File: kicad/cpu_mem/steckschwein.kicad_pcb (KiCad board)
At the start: 2 copper layers, 160 x 100.3 mm, 33 parts, among them P1 CONN_02X04, P3 CONN_01X03, P4 CONN_02X02, P5 CONN_02X25, SW1 SW_PUSH, U1 W65C02SP, U2 LM555N, U3 74HCT00, U4 74LS393, U5 GAL22V10, U6 28C256, U7 HM62256BLP-7, U8 HM62256BLP-7, U9 74LS139, X1 OSC

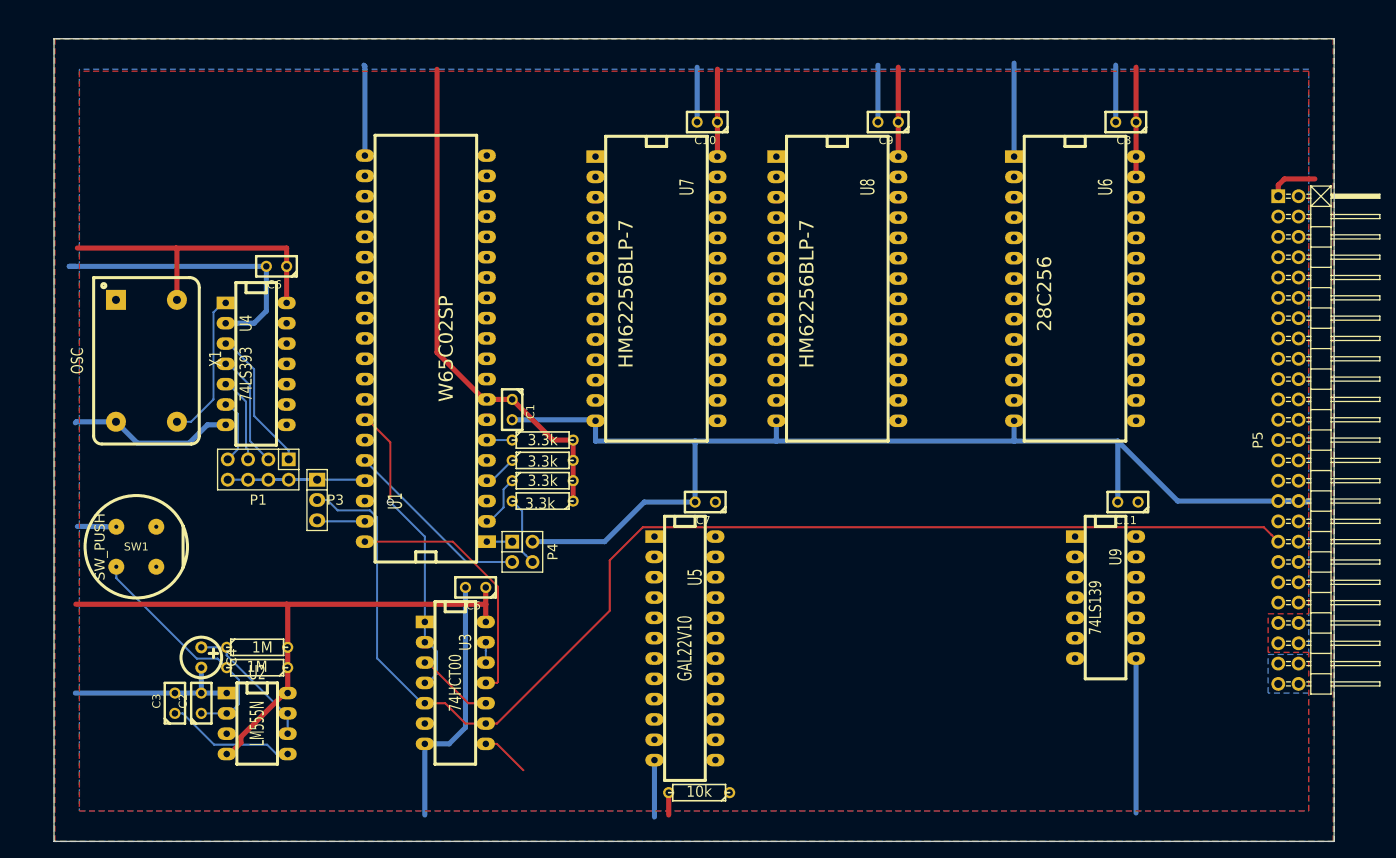
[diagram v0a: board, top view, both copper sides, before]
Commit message: new with new empty pcb
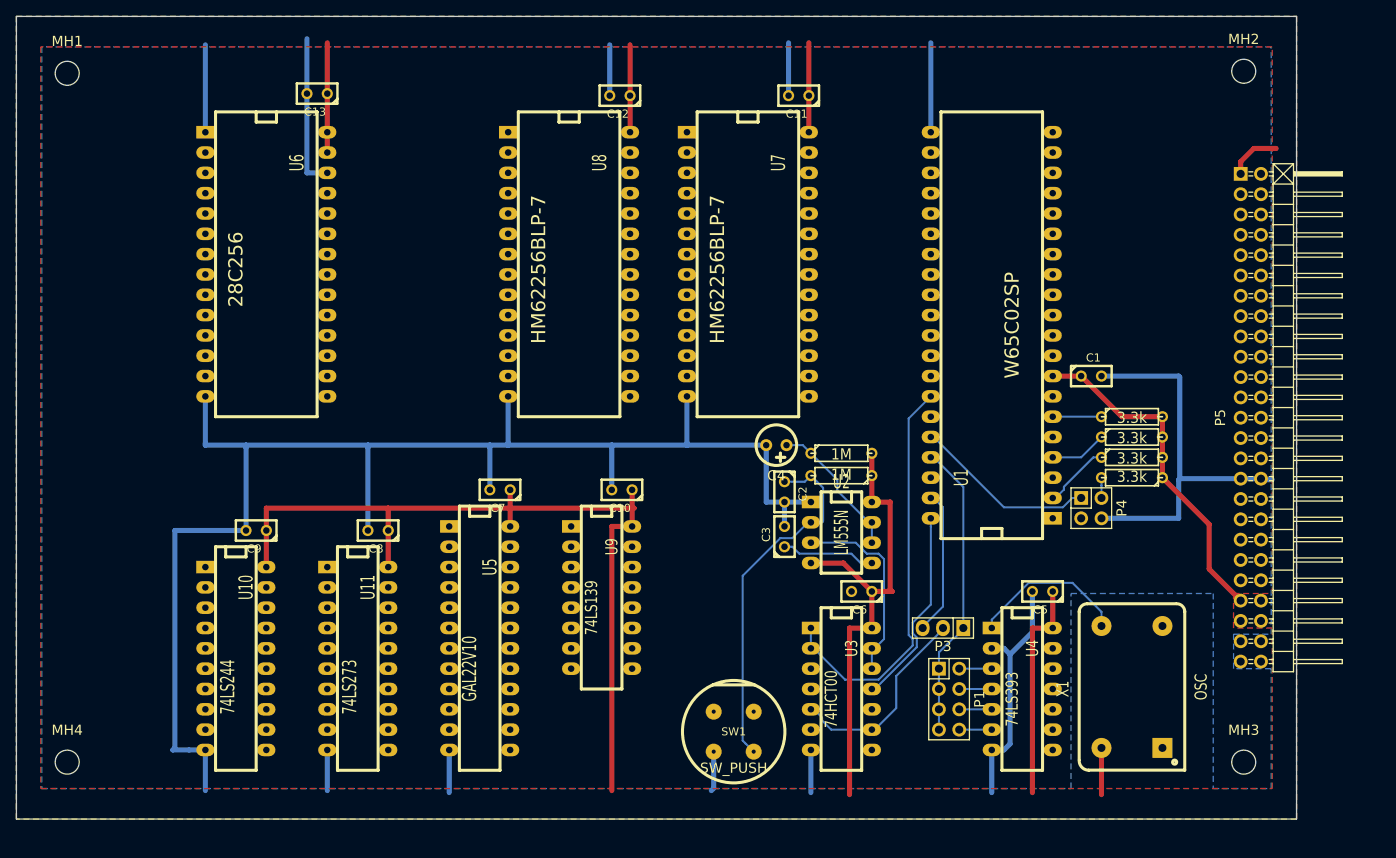
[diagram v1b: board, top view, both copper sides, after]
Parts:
- removed R8: 10k, Discret:R3
- added C12: 100n, Discret:C1, F.Cu at (137.7, 55.6)
- added C13: 100n, Discret:C1, F.Cu at (99.8, 55.4)
- added MH1: MountingHole_3mm_RevA_Date21Jun2010, Mounting_Holes:MountingHole_3mm, F.Cu at (68.6, 52.8)
- added MH2: MountingHole_3mm_RevA_Date21Jun2010, Mounting_Holes:MountingHole_3mm, F.Cu at (215.6, 52.6)
- added MH3: MountingHole_3mm_RevA_Date21Jun2010, Mounting_Holes:MountingHole_3mm, F.Cu at (215.6, 138.9)
- added MH4: MountingHole_3mm_RevA_Date21Jun2010, Mounting_Holes:MountingHole_3mm, F.Cu at (68.6, 138.9)
- added U10: 74LS244, Sockets_DIP:DIP-20__300_ELL, F.Cu at (89.7, 126.0)
- added U11: 74LS273, Sockets_DIP:DIP-20__300_ELL, F.Cu at (104.9, 126.0)
- U9: footprint Sockets_DIP:DIP-14__300_ELL -> Sockets_DIP:DIP-16__300_ELL
- moved X1 129.8 mm to (201.7, 129.5), turned to 90 degrees
- moved C8 106.5 mm to (107.4, 110.0)
- moved U4 104.0 mm to (188.0, 129.8)
- moved U6 101.1 mm to (93.5, 76.7)
- moved C9 94.1 mm to (92.2, 110.0)
- moved P1 91.0 mm to (178.8, 131.1), turned to 270 degrees
- moved C6 83.7 mm to (167.9, 117.6)
- moved P3 79.9 mm to (178.1, 122.2), turned to 180 degrees
- moved C3 79.0 mm to (158.2, 110.7)
- moved SW1 78.2 mm to (151.9, 135.1), turned to 180 degrees
- moved C2 77.5 mm to (158.2, 105.2), turned to 270 degrees
- moved R6 76.9 mm to (165.4, 100.3)
- moved R5 76.9 mm to (165.4, 103.1)
- moved U2 76.8 mm to (165.4, 110.2)
- moved C4 76.6 mm to (157.2, 99.3), turned to 180 degrees
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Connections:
- net /A10 renamed /decoder/A10
- net /A11 renamed /decoder/A11
- net /A12 renamed /decoder/A12
- net /A13 renamed /decoder/A13
- net /A14 renamed /decoder/A14
- net /A15 renamed /decoder/A15
- net /A6 renamed /decoder/A6
- net /A7 renamed /decoder/A7
- net /A8 renamed /decoder/A8
- net /A9 renamed /decoder/A9
- net /CS_HIRAM renamed /decoder//CS_HIRAM
- net /CS_LORAM renamed /decoder//CS_LORAM
- P1 pad 2: PH0-IN -> Net-(P1-Pad2)
- P1 pad 3: Net-(P1-Pad3) -> Net-(P1-Pad1)
- P1 pad 4: PH0-IN -> Net-(P1-Pad4)
- P1 pad 5: Net-(P1-Pad5) -> Net-(P1-Pad1)
- P1 pad 6: PH0-IN -> Net-(P1-Pad6)
- P1 pad 7: Net-(P1-Pad7) -> Net-(P1-Pad1)
- P1 pad 8: PH0-IN -> Net-(P1-Pad8)
- P3 pad 1: PH0-IN -> Net-(P1-Pad1)
- P4 pad 2: GND -> Net-(P4-Pad2)
- P4 pad 4: Net-(P4-Pad4) -> GND
- P5 pad 14: Net-(P5-Pad14) -> (no net)
- P5 pad 16: Net-(P5-Pad16) -> (no net)
- P5 pad 18: Net-(P5-Pad18) -> (no net)
- P5 pad 19: /CS_IO1 -> /CS_IO2
- P5 pad 20: /CS_IO0 -> /CS_IO1
- P5 pad 21: /CS_SND -> /CS_IO0
- P5 pad 36: Net-(P5-Pad36) -> (no net)
- P5 pad 37: Net-(P5-Pad37) -> (no net)
- P5 pad 38: Net-(P5-Pad38) -> (no net)
- P5 pad 39: Net-(P5-Pad39) -> (no net)
- P5 pad 40: Net-(P5-Pad40) -> (no net)
- P5 pad 41: Net-(P5-Pad41) -> (no net)
- P5 pad 42: Net-(P5-Pad42) -> (no net)
- P5 pad 5: /ROMOFF -> (no net)
- R4 pad 2: Net-(P4-Pad4) -> Net-(P4-Pad2)
- U1 pad 1: Net-(P4-Pad1) -> Net-(P4-Pad3)
- U1 pad 3: Net-(U1-Pad3) -> (no net)
- U1 pad 35: Net-(U1-Pad35) -> (no net)
- U1 pad 36: Net-(P4-Pad3) -> Net-(P4-Pad1)
- U1 pad 37: PH0-IN -> Net-(P1-Pad1)
- U1 pad 38: Net-(U1-Pad38) -> (no net)
- U1 pad 5: Net-(U1-Pad5) -> (no net)
- U1 pad 7: Net-(U1-Pad7) -> (no net)
- U4 pad 3: Net-(P1-Pad1) -> Net-(P1-Pad2)
- U4 pad 4: Net-(P1-Pad3) -> Net-(P1-Pad4)
- U4 pad 5: Net-(P1-Pad5) -> Net-(P1-Pad6)
- U4 pad 6: Net-(P1-Pad7) -> Net-(P1-Pad8)
- U5 pad 15: /ROMOFF -> Net-(U11-Pad2)
- U5 pad 16: /CS_ROM -> (no net)
- U5 pad 22: /CS_SND -> Net-(U10-Pad1)
- U5 pad 23: /CS_IO -> Net-(U5-Pad23)
- U6 pad 20: /CS_ROM -> (no net)
- U9 pad 1: /CS_IO -> (no net)
- U9 pad 10: (no net) -> /CS_IO2
- U9 pad 11: (no net) -> /CS_IO1
- U9 pad 12: (no net) -> /CS_IO0
- U9 pad 13: (no net) -> /Connector/A5
- U9 pad 14: (no net) -> /Connector/A4
- U9 pad 2: /Connector/A0 -> (no net)
- U9 pad 3: /Connector/A1 -> (no net)
- U9 pad 4: /CS_IO0 -> (no net)
- U9 pad 5: /CS_IO1 -> (no net)
- U9 pad 6: /CS_IO2 -> (no net)
- U9 pad 7: /CS_IO3 -> (no net)
- X1 pad 1: Net-(X1-Pad1) -> (no net)
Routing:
- net PHI2: track 156.6 -> 25.5 mm
- net VCC: track 227.1 -> 284.0 mm
- net PH0-IN: track 35.5 -> 0.00 mm
- net Net-(P4-Pad3): track 23.7 -> 0.00 mm
- net Net-(U2-Pad3): track 2.54 -> 24.5 mm
- net Net-(P1-Pad1): track 17.9 -> 39.8 mm
- net Net-(P4-Pad1): track 3.17 -> 22.9 mm
- net Net-(C2-Pad1): track 30.2 -> 45.4 mm
- net Net-(P1-Pad3): track 14.4 -> 0.00 mm
- net /RW: track 37.9 -> 51.2 mm, vias 1 -> 0
- net Net-(P3-Pad3): track 6.02 -> 18.1 mm
- net Net-(P1-Pad5): track 10.8 -> 0.00 mm
- net Net-(U3-Pad10): track 9.72 -> 0.00 mm
- net Net-(P4-Pad4): track 8.67 -> 0.00 mm
- net Net-(P1-Pad7): track 8.22 -> 0.00 mm
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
